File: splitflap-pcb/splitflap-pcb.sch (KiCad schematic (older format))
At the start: 23 parts, among them J1 INPUT CONN, J2 HALL 1, J3 HALL 2, J4 STEPPER 1, J5 STEPPER 2, J6 OUTPUT CONN, J7 AVR-ISP-6, U1 NCV78M05, U2 ATtiny88-AU, U3 TPIC6595

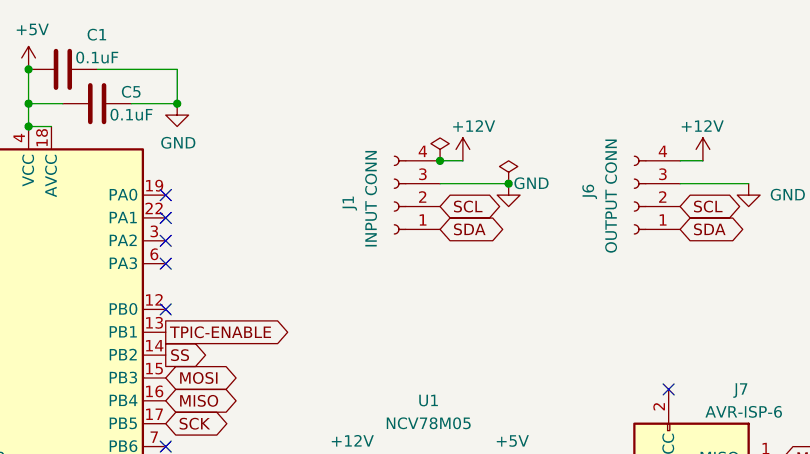
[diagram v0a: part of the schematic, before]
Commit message: v09
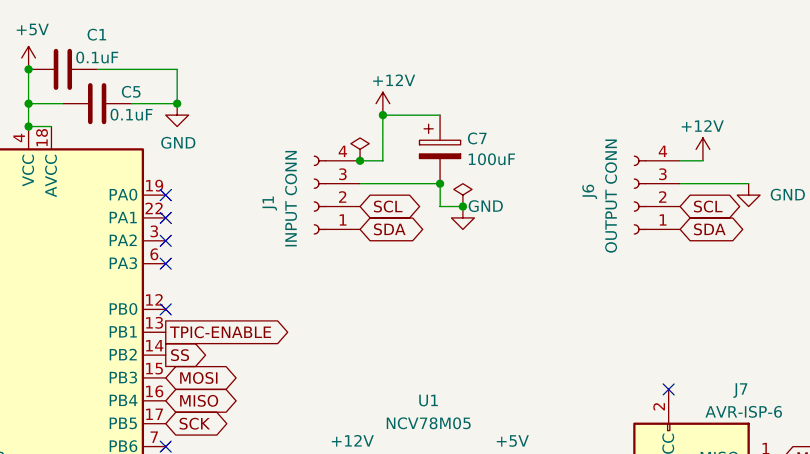
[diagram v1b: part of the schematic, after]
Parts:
- added C7: 100uF, Capacitor_THT:CP_Radial_D6.3mm_P2.50mm, symbol Device:CP
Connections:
- net +12V: now also C7.1
- net GND: now also C7.2
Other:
- moved on the sheet: J1
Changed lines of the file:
@@
 L Connector:Conn_01x04_Female J1
 U 1 1 5CC15B7D
-P 3900 1900
-F 0 "J1" V 4100 1850 50  0000 L CNN
-F 1 "INPUT CONN" V 4000 1650 50  0000 L CNN
-F 2 "splitflap-pcb:TE_640456-4" H 3900 1900 50  0001 C CNN
-F 3 "~" H 3900 1900 50  0001 C CNN
-	1    3900 1900
+P 3550 1900
+F 0 "J1" V 3750 1850 50  0000 L CNN
+F 1 "INPUT CONN" V 3650 1650 50  0000 L CNN
+F 2 "splitflap-pcb:TE_640456-4" H 3550 1900 50  0001 C CNN
+F 3 "~" H 3550 1900 50  0001 C CNN
+	1    3550 1900
 	-1   0    0    1
 $EndComp
-Text GLabel 4100 1900 2    50   BiDi ~ 0
+Text GLabel 3750 1900 2    50   BiDi ~ 0
 SCL
-Text GLabel 4100 2000 2    50   BiDi ~ 0
+Text GLabel 3750 2000 2    50   BiDi ~ 0
 SDA
 Text GLabel 5150 1900 2    50   BiDi ~ 0
@@
 L power:GND #PWR0101
 U 1 1 5CC88AAA
-P 4400 1800
-F 0 "#PWR0101" H 4400 1550 50  0001 C CNN
-F 1 "GND" H 4500 1800 50  0000 C CNN
-F 2 "" H 4400 1800 50  0001 C CNN
-F 3 "" H 4400 1800 50  0001 C CNN
-	1    4400 1800
+P 4200 1900
+F 0 "#PWR0101" H 4200 1650 50  0001 C CNN
+F 1 "GND" H 4300 1900 50  0000 C CNN
+F 2 "" H 4200 1900 50  0001 C CNN
+F 3 "" H 4200 1900 50  0001 C CNN
+	1    4200 1900
 	1    0    0    -1
 $EndComp
@@
 L power:PWR_FLAG #FLG0101
 U 1 1 5CC8C3CC
-P 4100 1700
-F 0 "#FLG0101" H 4100 1775 50  0001 C CNN
-F 1 "PWR_FLAG" H 3950 1850 50  0001 C CNN
-F 2 "" H 4100 1700 50  0001 C CNN
-F 3 "~" H 4100 1700 50  0001 C CNN
-	1    4100 1700
+P 3750 1700
+F 0 "#FLG0101" H 3750 1775 50  0001 C CNN
+F 1 "PWR_FLAG" H 3600 1850 50  0001 C CNN
+F 2 "" H 3750 1700 50  0001 C CNN
+F 3 "~" H 3750 1700 50  0001 C CNN
+	1    3750 1700
 	1    0    0    -1
 $EndComp
@@
 L power:PWR_FLAG #FLG0102
 U 1 1 5CC8CDF8
-P 4400 1800
-F 0 "#FLG0102" H 4400 1875 50  0001 C CNN
-F 1 "PWR_FLAG" H 4650 1900 50  0001 C CNN
-F 2 "" H 4400 1800 50  0001 C CNN
-F 3 "~" H 4400 1800 50  0001 C CNN
-	1    4400 1800
+P 4200 1900
+F 0 "#FLG0102" H 4200 1975 50  0001 C CNN
+F 1 "PWR_FLAG" H 4450 2000 50  0001 C CNN
+F 2 "" H 4200 1900 50  0001 C CNN
+F 3 "~" H 4200 1900 50  0001 C CNN
+	1    4200 1900
 	1    0    0    -1
 $EndComp
@@
 L power:+12V #PWR02
 U 1 1 5CC3B088
-P 4200 1700
-F 0 "#PWR02" H 4200 1550 50  0001 C CNN
-F 1 "+12V" H 4150 1850 50  0000 L CNN
-F 2 "" H 4200 1700 50  0001 C CNN
-F 3 "" H 4200 1700 50  0001 C CNN
-	1    4200 1700
-	1    0    0    -1
-$EndComp
-Connection ~ 4400 1800
-Wire Wire Line
-	4100 1700 4200 1700
-Connection ~ 4100 1700
+P 3850 1500
+F 0 "#PWR02" H 3850 1350 50  0001 C CNN
+F 1 "+12V" H 3800 1650 50  0000 L CNN
+F 2 "" H 3850 1500 50  0001 C CNN
+F 3 "" H 3850 1500 50  0001 C CNN
+	1    3850 1500
+	1    0    0    -1
+$EndComp
+Wire Wire Line
+	3750 1700 3850 1700
+Connection ~ 3750 1700
 Text GLabel 6050 1950 3    50   BiDi ~ 0
 SCL
@@
 Connection ~ 3700 3100
 Wire Wire Line
-	4100 1800 4400 1800
-Wire Wire Line
 	2900 3850 3000 3850
 Wire Wire Line
@@
 Connection ~ 2950 1450
 Connection ~ 2300 1300
+Wire Wire Line
+	3850 1500 4100 1500
+Wire Wire Line
+	3850 1700 3850 1500
+Connection ~ 3850 1500
+Wire Wire Line
+	3750 1800 4100 1800
+Wire Wire Line
+	4100 1800 4100 1900
+Wire Wire Line
+	4100 1900 4200 1900
+Connection ~ 4200 1900
+$Comp
+L Device:CP C7
+U 1 1 5CCC6205
+P 4100 1650
+F 0 "C7" H 4218 1696 50  0000 L CNN
+F 1 "100uF" H 4218 1605 50  0000 L CNN
+F 2 "Capacitor_THT:CP_Radial_D6.3mm_P2.50mm" H 4138 1500 50  0001 C CNN
+F 3 "~" H 4100 1650 50  0001 C CNN
+	1    4100 1650
+	1    0    0    -1
+$EndComp
+Connection ~ 4100 1800
 $EndSCHEMATC
